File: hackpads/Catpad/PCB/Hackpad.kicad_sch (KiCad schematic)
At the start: 63 parts, among them J1 Conn_01x04, J2 Conn_01x04, SW1 SW_SPST, SW10 SW_SPST, SW11 SW_SPST, SW12 SW_SPST, SW13 SW_SPST, SW14 SW_SPST, SW15 SW_SPST, SW16 SW_SPST, SW17 SW_SPST, SW18 SW_SPST, SW19 SW_SPST, SW2 SW_SPST, SW20 SW_SPST, SW3 SW_SPST, SW4 SW_SPST, SW5 SW_SPST, SW6 SW_SPST, SW7 SW_SPST, SW8 SW_SPST, SW9 SW_SPST, U1 Seeed Studio XIAO SAMD21

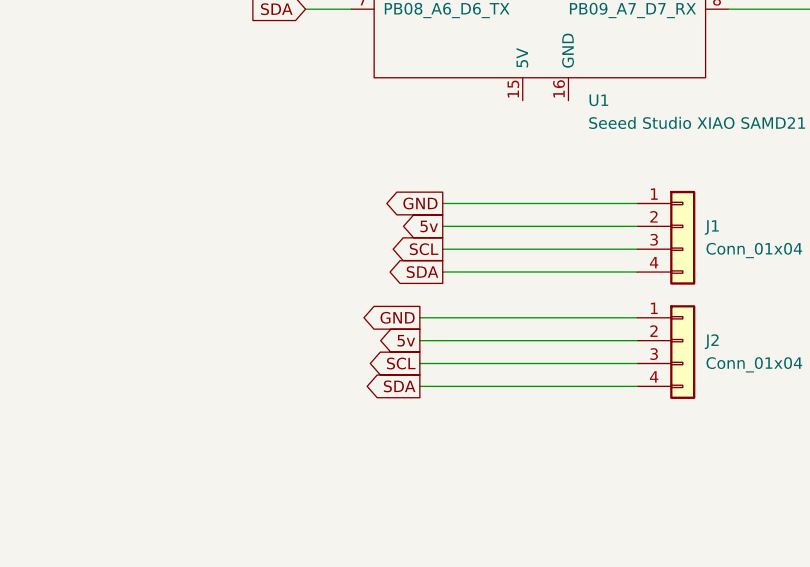
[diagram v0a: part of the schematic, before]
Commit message: fixed stuff
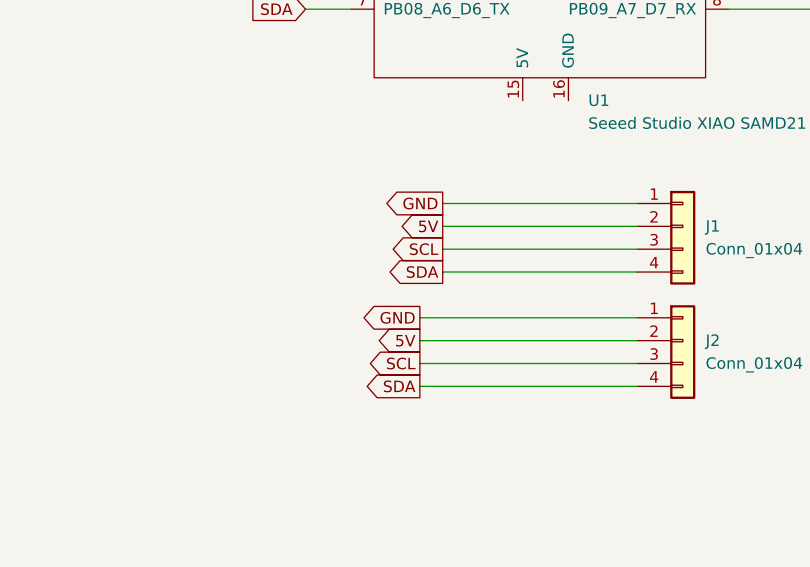
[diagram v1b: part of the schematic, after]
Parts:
- D1, D22, D23, D24, D25, D26, D27, D28, D29, D30, D31, D32, D33, D34, D35, D36, D37, D38, D39, D40: footprint LED_SMD:LED_0603_1608Metric_Pad1.05x0.95mm_HandSolder -> LED_SMD:LED_1206_3216Metric
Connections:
- net 5v is gone; now on net 5V: J1.2 (Pin_2), J2.2 (Pin_2)
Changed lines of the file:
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@@
 		)
 	)
-	(global_label "5v"
+	(global_label "5V"
 		(shape output)
 		(at 219.71 139.7 180)
@@
 		)
 		(property "Intersheetrefs" "${INTERSHEET_REFS}"
-			(at 214.5477 139.7 0)
+			(at 214.4267 139.7 0)
 			(effects
 				(font
@@
 		)
 	)
-	(global_label "5v"
+	(global_label "5V"
 		(shape output)
 		(at 222.25 127 180)
@@
 		)
 		(property "Intersheetrefs" "${INTERSHEET_REFS}"
-			(at 217.0877 127 0)
+			(at 216.9667 127 0)
 			(effects
 				(font
@@
 			)
 		)
-		(property "Footprint" "LED_SMD:LED_0603_1608Metric_Pad1.05x0.95mm_HandSolder"
+		(property "Footprint" "LED_SMD:LED_1206_3216Metric"
 			(at 179.07 58.42 0)
 			(effects
@@
 			)
 		)
-		(property "Footprint" "LED_SMD:LED_0603_1608Metric_Pad1.05x0.95mm_HandSolder"
+		(property "Footprint" "LED_SMD:LED_1206_3216Metric"
 			(at 179.07 35.56 0)
 			(effects
@@
 			)
 		)
-		(property "Footprint" "LED_SMD:LED_0603_1608Metric_Pad1.05x0.95mm_HandSolder"
+		(property "Footprint" "LED_SMD:LED_1206_3216Metric"
 			(at 179.07 73.66 0)
 			(effects
@@
 			)
 		)
-		(property "Footprint" "LED_SMD:LED_0603_1608Metric_Pad1.05x0.95mm_HandSolder"
+		(property "Footprint" "LED_SMD:LED_1206_3216Metric"
 			(at 179.07 77.47 0)
 			(effects
@@
 			)
 		)
-		(property "Footprint" "LED_SMD:LED_0603_1608Metric_Pad1.05x0.95mm_HandSolder"
+		(property "Footprint" "LED_SMD:LED_1206_3216Metric"
 			(at 179.07 20.32 0)
 			(effects
@@
 			)
 		)
-		(property "Footprint" "LED_SMD:LED_0603_1608Metric_Pad1.05x0.95mm_HandSolder"
+		(property "Footprint" "LED_SMD:LED_1206_3216Metric"
 			(at 179.07 81.28 0)
 			(effects
@@
 			)
 		)
-		(property "Footprint" "LED_SMD:LED_0603_1608Metric_Pad1.05x0.95mm_HandSolder"
+		(property "Footprint" "LED_SMD:LED_1206_3216Metric"
 			(at 179.07 66.04 0)
 			(effects
@@
 			)
 		)
-		(property "Footprint" "LED_SMD:LED_0603_1608Metric_Pad1.05x0.95mm_HandSolder"
+		(property "Footprint" "LED_SMD:LED_1206_3216Metric"
 			(at 179.07 24.13 0)
 			(effects
@@
 			)
 		)
-		(property "Footprint" "LED_SMD:LED_0603_1608Metric_Pad1.05x0.95mm_HandSolder"
+		(property "Footprint" "LED_SMD:LED_1206_3216Metric"
 			(at 179.07 50.8 0)
 			(effects
@@
 			)
 		)
-		(property "Footprint" "LED_SMD:LED_0603_1608Metric_Pad1.05x0.95mm_HandSolder"
+		(property "Footprint" "LED_SMD:LED_1206_3216Metric"
 			(at 179.07 31.75 0)
 			(effects
@@
 			)
 		)
-		(property "Footprint" "LED_SMD:LED_0603_1608Metric_Pad1.05x0.95mm_HandSolder"
+		(property "Footprint" "LED_SMD:LED_1206_3216Metric"
 			(at 179.07 39.37 0)
 			(effects
@@
 			)
 		)
-		(property "Footprint" "LED_SMD:LED_0603_1608Metric_Pad1.05x0.95mm_HandSolder"
+		(property "Footprint" "LED_SMD:LED_1206_3216Metric"
 			(at 179.07 27.94 0)
 			(effects
@@
 			)
 		)
-		(property "Footprint" "LED_SMD:LED_0603_1608Metric_Pad1.05x0.95mm_HandSolder"
+		(property "Footprint" "LED_SMD:LED_1206_3216Metric"
 			(at 179.07 69.85 0)
 			(effects
@@
 			)
 		)
-		(property "Footprint" "LED_SMD:LED_0603_1608Metric_Pad1.05x0.95mm_HandSolder"
+		(property "Footprint" "LED_SMD:LED_1206_3216Metric"
 			(at 179.07 12.7 0)
 			(effects
@@
 			)
 		)
-		(property "Footprint" "LED_SMD:LED_0603_1608Metric_Pad1.05x0.95mm_HandSolder"
+		(property "Footprint" "LED_SMD:LED_1206_3216Metric"
 			(at 179.07 62.23 0)
 			(effects
@@
 			)
 		)
-		(property "Footprint" "LED_SMD:LED_0603_1608Metric_Pad1.05x0.95mm_HandSolder"
+		(property "Footprint" "LED_SMD:LED_1206_3216Metric"
 			(at 179.07 43.18 0)
 			(effects
@@
 			)
 		)
-		(property "Footprint" "LED_SMD:LED_0603_1608Metric_Pad1.05x0.95mm_HandSolder"
+		(property "Footprint" "LED_SMD:LED_1206_3216Metric"
 			(at 179.07 54.61 0)
 			(effects
@@
 			)
 		)
-		(property "Footprint" "LED_SMD:LED_0603_1608Metric_Pad1.05x0.95mm_HandSolder"
+		(property "Footprint" "LED_SMD:LED_1206_3216Metric"
 			(at 179.07 85.09 0)
 			(effects
@@
 			)
 		)
-		(property "Footprint" "LED_SMD:LED_0603_1608Metric_Pad1.05x0.95mm_HandSolder"
+		(property "Footprint" "LED_SMD:LED_1206_3216Metric"
 			(at 179.07 46.99 0)
 			(effects
@@
 			)
 		)
-		(property "Footprint" "LED_SMD:LED_0603_1608Metric_Pad1.05x0.95mm_HandSolder"
+		(property "Footprint" "LED_SMD:LED_1206_3216Metric"
 			(at 179.07 16.51 0)
 			(effects
